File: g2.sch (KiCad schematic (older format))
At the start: 85 parts, among them J1 USB_B_Micro, J10 Screw, J11 Screw, J12 A, J13 Micro, J14 Speaker, J15 A, J16 A, J17 i2c, J18 i2c, J19 Micro, J2 Screw_Terminal_01x04, J20 Micro, J21 Conn_02x04_Odd_Even, J22 Conn_01x02_Male, J23 i2c, J24 A, J25 A, J3 Screw, J4 pwm, J5 pwm, J6 pwm, J7 Screw, J8 Screw, J9 Screw, K1 SRD, K2 SRD, K3 SRD, K4 SRD, K5 SRD, K6 SRD, Q1 2N3904, Q2 2N3904, Q3 2N3904, Q4 2N3904, Q5 2N3904, Q6 2N3904, U1 PC817, U2 PC817, U3 PC817, U4 ATmega328P-PU, U5 Sim800l, U6 PC817, U7 PC817, U8 PC817, U9 LD1117S33TR_SOT223, Y1 Crystal

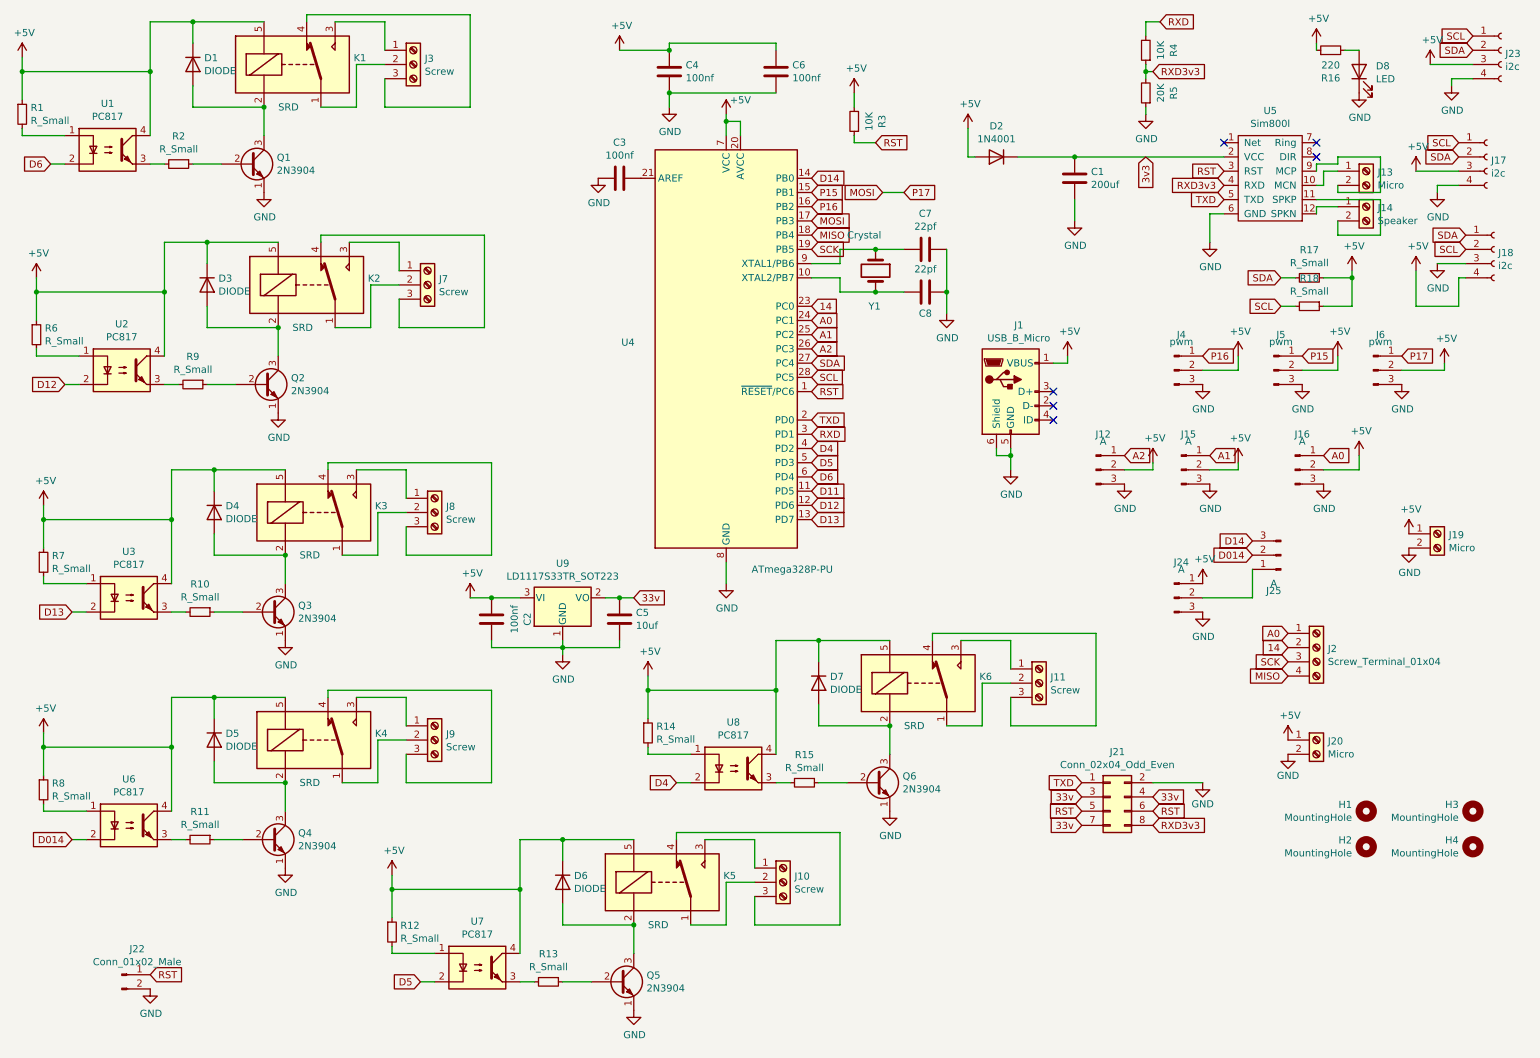
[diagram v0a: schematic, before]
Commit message: final
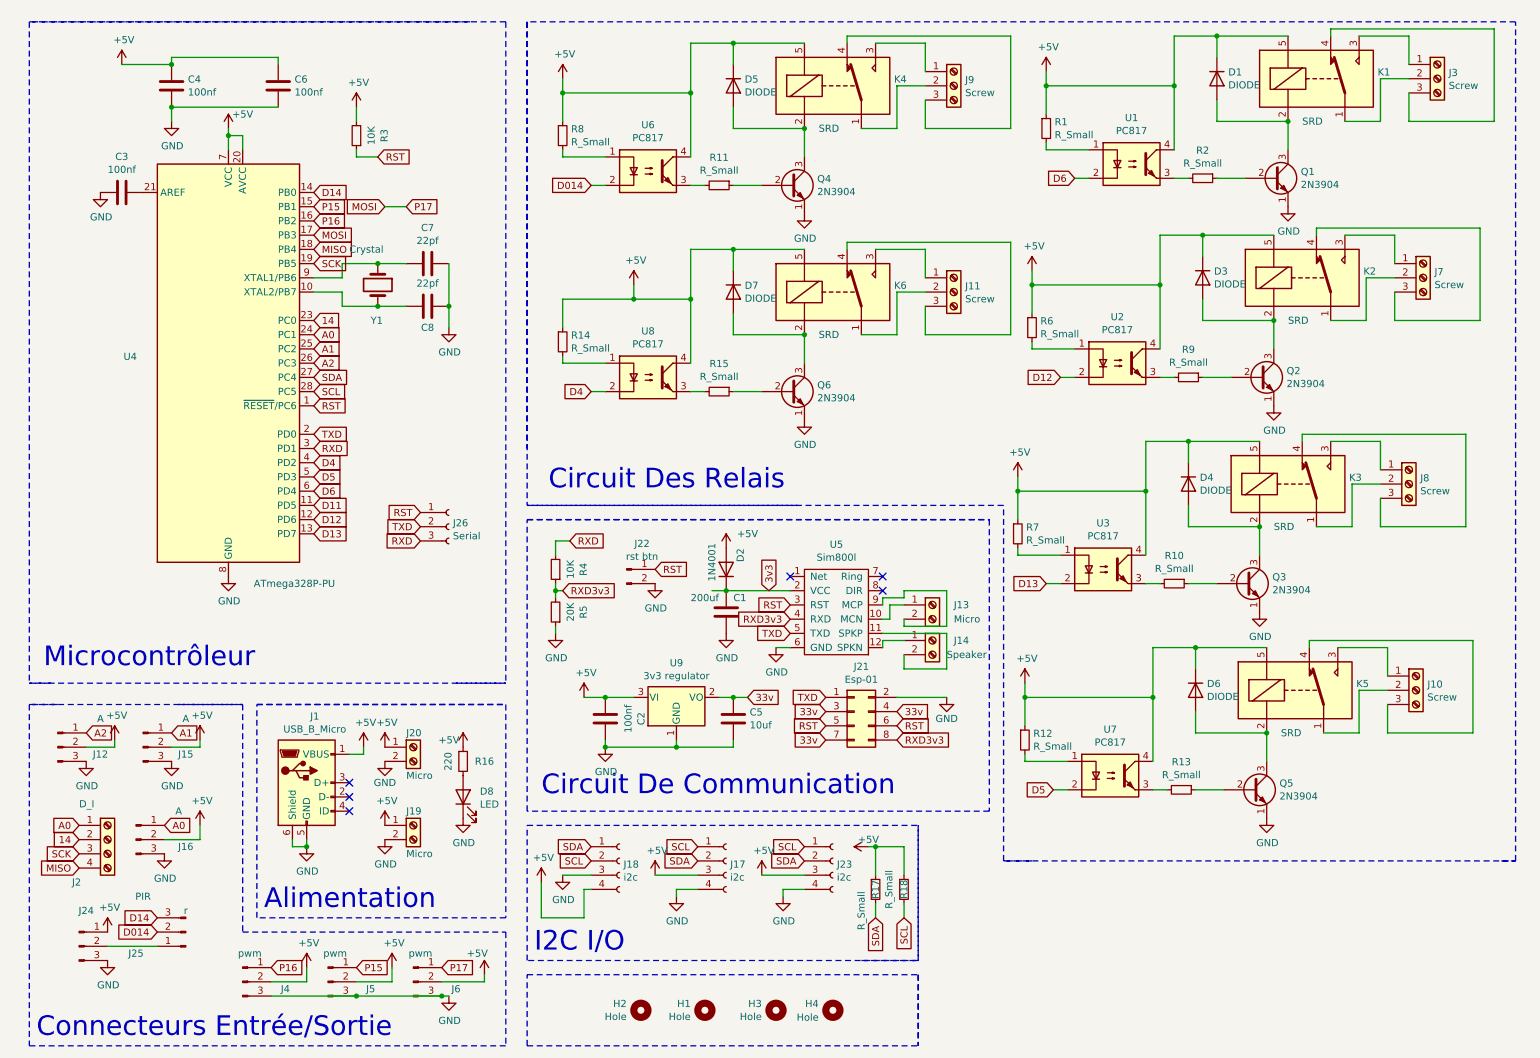
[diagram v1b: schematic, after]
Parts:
- added J26: Serial, Connector_PinSocket_2.54mm:PinSocket_1x03_P2.54mm_Vertical, symbol Connector:Conn_01x03_Female
- H1, H2, H3, H4: value MountingHole -> Hole
- J2: value Screw_Terminal_01x04 -> D_I
- J21: value Conn_02x04_Odd_Even -> Esp-01
- J22: value Conn_01x02_Male -> rst btn
- J24: value A -> PIR
- J25: value A -> r
- U9: value LD1117S33TR_SOT223 -> 3v3 regulator
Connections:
- net RST: now also J26.1 (Pin_1)
- net RXD: now also J26.3 (Pin_3)
- net TXD: now also J26.2 (Pin_2)
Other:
- note added: "Alimentation"
- note added: "Circuit De Communication"
- note added: "Circuit Des Relais"
- note added: "Connecteurs Entrée/Sortie"
- note added: "I2C I/O"
- note added: "Microcontrôleur"
- moved on the sheet: C1, C2, C3, C4, C5, C6, C7, C8, D1, D2, D3, D4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
